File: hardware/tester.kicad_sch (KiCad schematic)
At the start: 4 parts, among them SW7 SW_DIP_x08

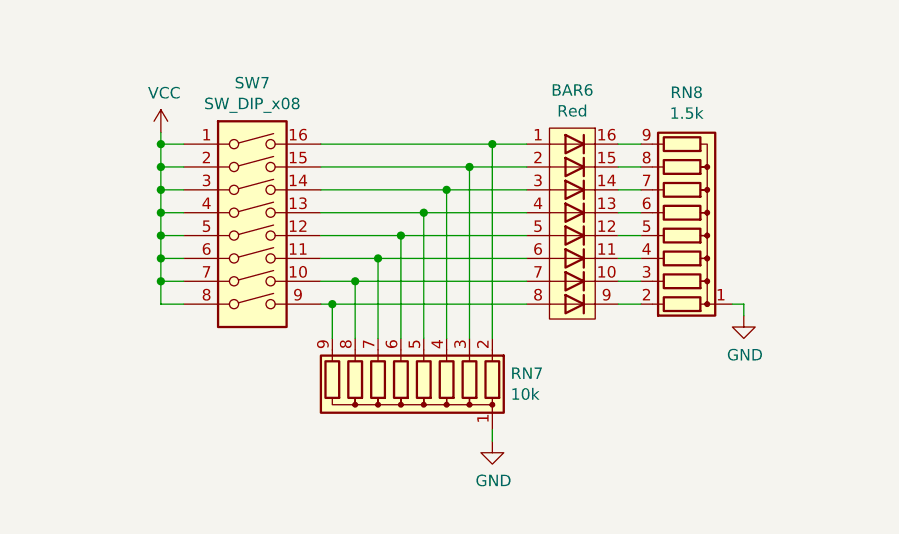
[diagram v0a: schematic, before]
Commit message: FIx tester
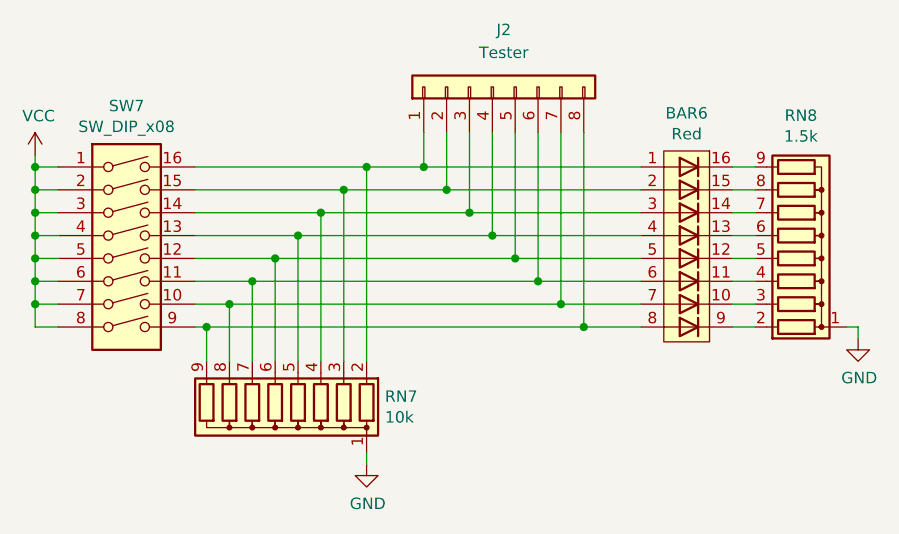
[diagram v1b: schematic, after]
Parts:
- added J2: Tester, symbol Connector_Generic:Conn_01x08
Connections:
- net at BAR6.1 (A), RN7.2 (R1), SW7.16: now also J2.1 (Pin_1)
- net at BAR6.2 (A), RN7.3 (R2), SW7.15: now also J2.2 (Pin_2)
- net at BAR6.3 (A), RN7.4 (R3), SW7.14: now also J2.3 (Pin_3)
- net at BAR6.4 (A), RN7.5 (R4), SW7.13: now also J2.4 (Pin_4)
- net at BAR6.5 (A), RN7.6 (R5), SW7.12: now also J2.5 (Pin_5)
- net at BAR6.6 (A), RN7.7 (R6), SW7.11: now also J2.6 (Pin_6)
- net at BAR6.7 (A), RN7.8 (R7), SW7.10: now also J2.7 (Pin_7)
- net at BAR6.8 (A), RN7.9 (R8), SW7.9: now also J2.8 (Pin_8)
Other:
- moved on the sheet: BAR6, RN7, RN8, SW7
